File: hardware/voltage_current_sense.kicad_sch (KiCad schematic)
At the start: 32 parts, among them J11 Conn_01x02, U10 NME0505SC, U11 LM324, U6 INA126U/2K5, U8 LTC6992CS6-2-TRMPBF, U9 6N137

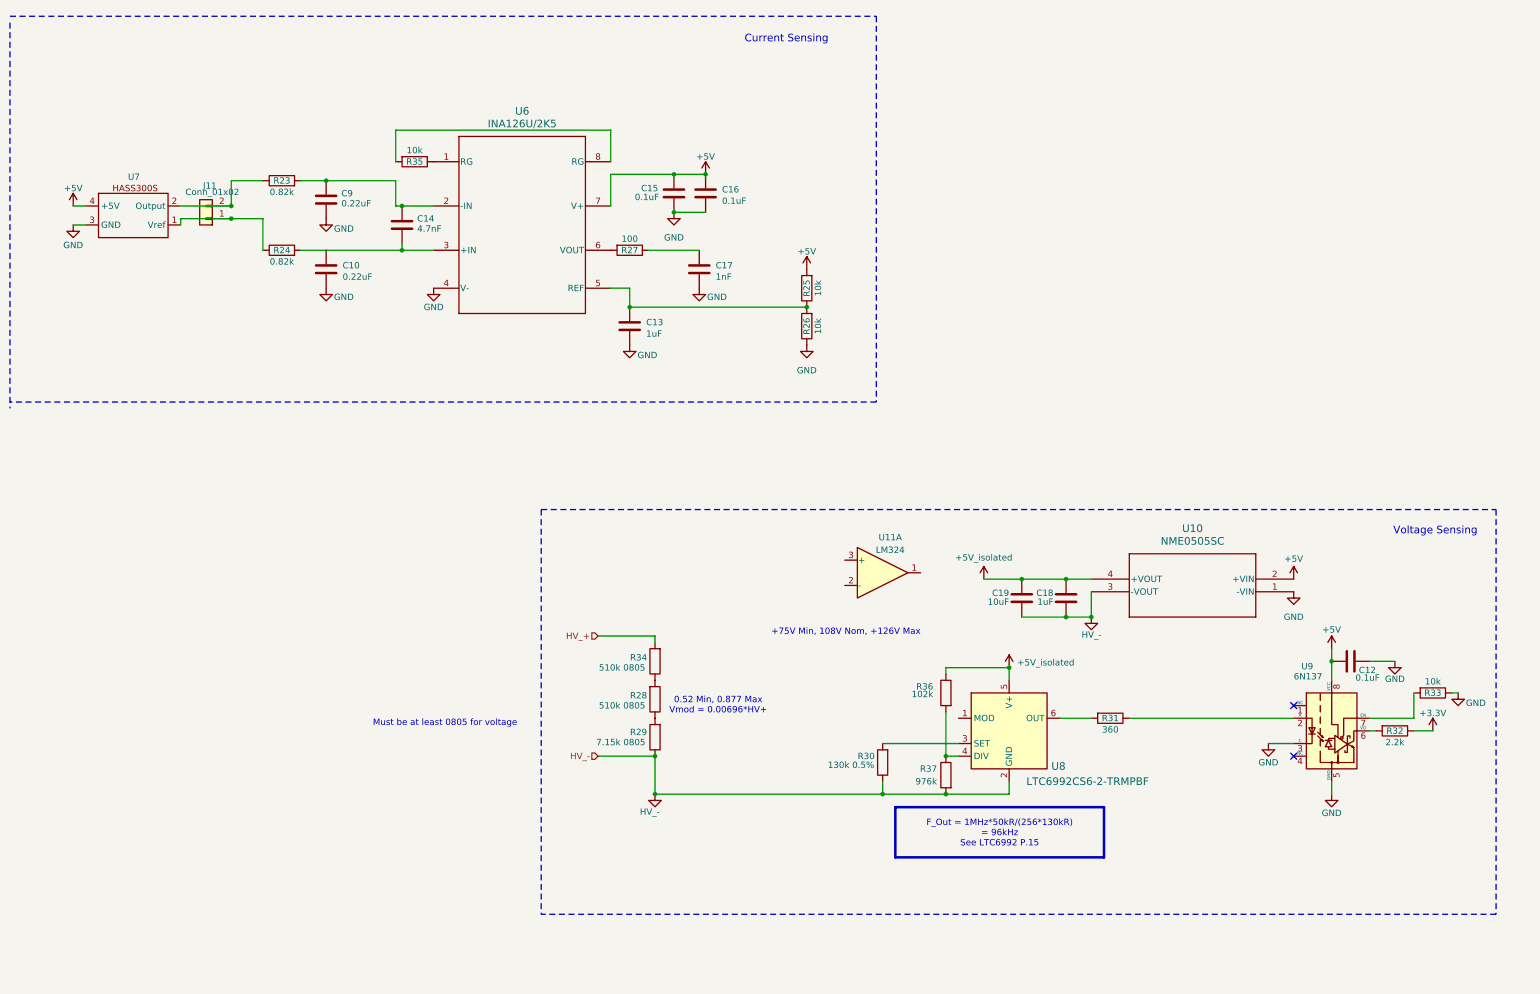
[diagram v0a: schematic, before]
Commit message: adding connectors
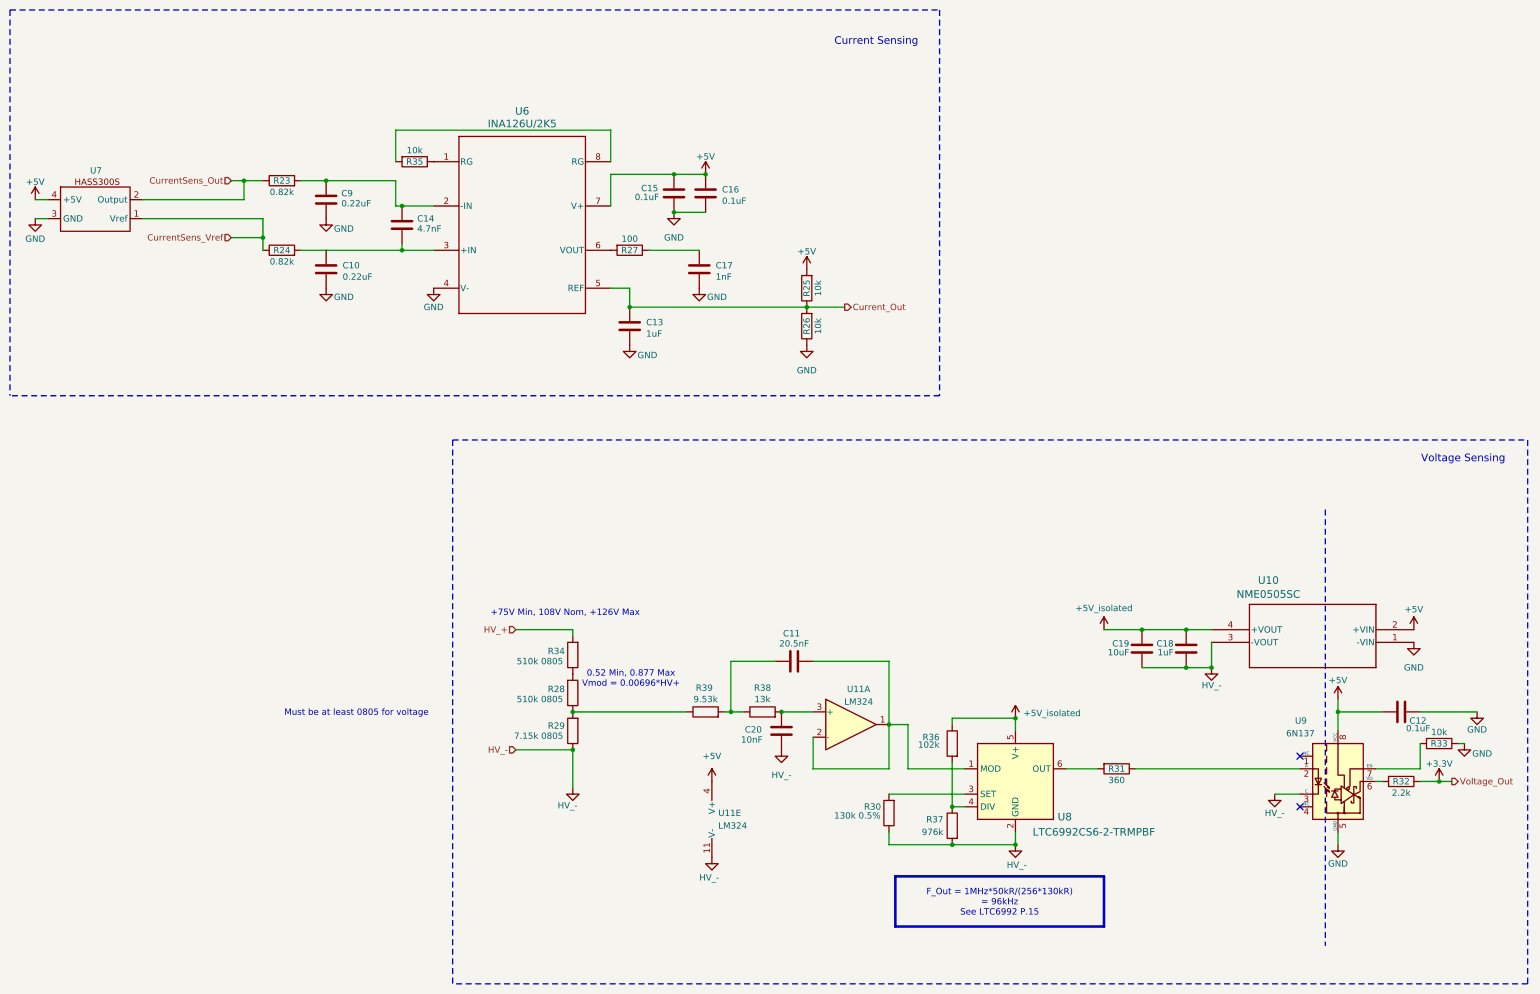
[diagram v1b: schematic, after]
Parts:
- removed J11: Conn_01x02, symbol Connector_Generic:Conn_01x02
- added C11: 20.5nF, symbol Device:C
- added C20: 10nF, symbol Device:C
- added R38: 13k, symbol Device:R
- added R39: 9.53k, symbol Device:R
- added unit 5 of U11
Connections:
- net +5V: now also U11.4 (V+)
- net GND: no longer U9.3 (C)
- net HV_-: now also U9.3 (C), C20.1, U11.11 (V-)
- net CurrentSens_Vref: now reaches R24.1, U7.1 (Vref)
- net CurrentSens_Out: now reaches R23.1, U7.2 (Output)
- net at U8.1 (MOD): now also U11.1, U11.2 (-), C11.2
- net Current_Out: now reaches C13.1, R25.1, R26.2, U6.5 (REF)
- net at R28.1, R29.2: now also R39.1
- net at U11.3 (+): now also C20.2, R38.2
- new net: C11.1, R38.1, R39.2
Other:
- moved on the sheet: C12, C18, C19, R28, R29, R30, R31, R32, R33, R34, R36, R37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
